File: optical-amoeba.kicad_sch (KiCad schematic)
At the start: 5 parts, among them J1 Conn_01x08_Male, Q1 Q_Photo_NPN_CE

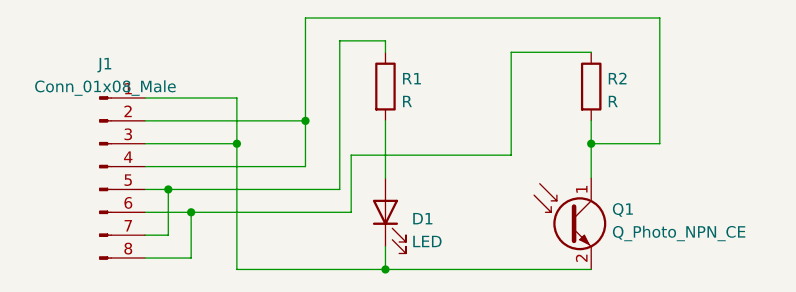
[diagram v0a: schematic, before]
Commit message: Add jlcpcb gerber and assembly files
M  OpticalSymbols_Library.kicad_sym
A  jlcpcb/gerber/optical-amoeba-B_Cu.gbl
A  jlcpcb/gerber/optical-amoeba-B_Mask.gbs
A  jlcpcb/gerber/optical-amoeba-B_Paste.gbp
A  jlcpcb/gerber/optical-amoeba-B_Silkscreen.gbo
A  jlcpcb/gerber/optical-amoeba-Edge_Cuts.gm1
A  jlcpcb/gerber/optical-amoeba-F_Cu.gtl
A  jlcpcb/gerber/optical-amoeba-F_Mask.gts
A  jlcpcb/gerber/optical-amoeba-F_Paste.gtp
A  jlcpcb/gerber/optical-amoeba-F_Silkscreen.gto
A  jlcpcb/gerber/optical-amoeba-NPTH-drl_map.gbr
A  jlcpcb/gerber/optical-amoeba-NPTH.drl
A  jlcpcb/gerber/optical-amoeba-PTH-drl_map.gbr
A  jlcpcb/gerber/optical-amoeba-PTH.drl
M  optical-amoeba.kicad_pcb
M  optical-amoeba.kicad_prl
M  optical-amoeba.kicad_sch
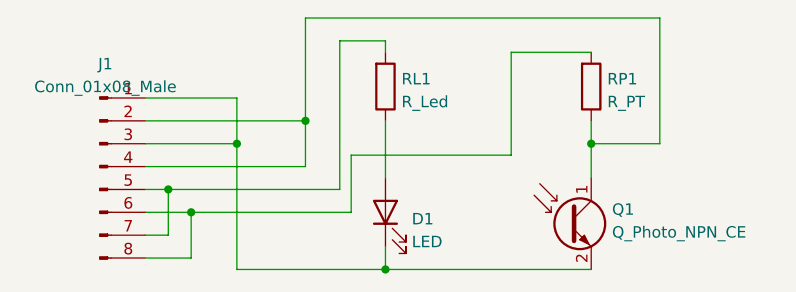
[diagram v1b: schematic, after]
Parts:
- removed R1: R, Resistor_SMD:R_0603_1608Metric, symbol Device:R
- removed R2: R, Resistor_SMD:R_0805_2012Metric, symbol Device:R
- added RL1: R_Led, Resistor_SMD:R_0603_1608Metric, symbol OpticalSymbols_Library:R_Led
- added RP1: R_PT, Resistor_SMD:R_0805_2012Metric, symbol OpticalSymbols_Library:R_PT
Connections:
- net at J1.2 (Pin_2), J1.4 (Pin_4), Q1.1 (C): now also RP1.2
- net at J1.5 (Pin_5), J1.7 (Pin_7): now also RL1.1
- net at J1.6 (Pin_6), J1.8 (Pin_8): now also RP1.1
- net at D1.2 (A): now also RL1.2
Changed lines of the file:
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@@
     (pin "8")
-  )
-  (symbol (lib_id "Device:R") (at 100.33 67.31 0) (unit 1)
-    (in_bom yes) (on_board yes) (fields_autoplaced)
-    (property "Reference" "R1" (id 0) (at 102.108 66.4753 0)
-      (effects (font (size 1.27 1.27)) (justify left))
-    )
-    (property "Value" "R" (id 1) (at 102.108 69.0122 0)
-      (effects (font (size 1.27 1.27)) (justify left))
-    )
-    (property "Footprint" "Resistor_SMD:R_0603_1608Metric" (id 2) (at 98.552 67.31 90)
-      (effects (font (size 1.27 1.27)) hide)
-    )
-    (property "Datasheet" "~" (id 3) (at 100.33 67.31 0)
-      (effects (font (size 1.27 1.27)) hide)
-    )
-    (property "JLC" "0603" (id 4) (at 100.33 67.31 0)
-      (effects (font (size 1.27 1.27)) hide)
-    )
-    (property "LCSC" "C4190" (id 5) (at 100.33 67.31 0)
-      (effects (font (size 1.27 1.27)) hide)
-    )
-    (pin "1")
-    (pin "2")
   )
   (symbol (lib_id "Device:Q_Photo_NPN_CE") (at 120.65 82.55 0) (unit 1)
@@
     (property "LCSC" "C264383" (id 5) (at 120.65 82.55 0)
       (effects (font (size 1.27 1.27)) hide)
+    )
+    (pin "1")
+    (pin "2")
+  )
+  (symbol (lib_id "OpticalSymbols_Library:R_PT") (at 123.19 67.31 0) (unit 1)
+    (in_bom yes) (on_board yes) (fields_autoplaced)
+    (property "Reference" "RP1" (id 0) (at 124.968 66.4753 0)
+      (effects (font (size 1.27 1.27)) (justify left))
+    )
+    (property "Value" "R_PT" (id 1) (at 124.968 69.0122 0)
+      (effects (font (size 1.27 1.27)) (justify left))
+    )
+    (property "Footprint" "Resistor_SMD:R_0805_2012Metric" (id 2) (at 124.46 73.66 90)
+      (effects (font (size 1.27 1.27)) (justify left) hide)
+    )
+    (property "Datasheet" "~" (id 3) (at 123.19 68.58 0)
+      (effects (font (size 1.27 1.27)) hide)
+    )
+    (property "JLC" "0805-2012" (id 4) (at 120.65 71.12 0)
+      (effects (font (size 0.5 0.5)) hide)
+    )
+    (property "LCSC" "C17713" (id 5) (at 127 63.5 0)
+      (effects (font (size 0.5 0.5)) hide)
+    )
+    (pin "1")
+    (pin "2")
+  )
+  (symbol (lib_id "OpticalSymbols_Library:R_Led") (at 100.33 67.31 0) (unit 1)
+    (in_bom yes) (on_board yes) (fields_autoplaced)
+    (property "Reference" "RL1" (id 0) (at 102.108 66.4753 0)
+      (effects (font (size 1.27 1.27)) (justify left))
+    )
+    (property "Value" "R_Led" (id 1) (at 102.108 69.0122 0)
+      (effects (font (size 1.27 1.27)) (justify left))
+    )
+    (property "Footprint" "Resistor_SMD:R_0603_1608Metric" (id 2) (at 101.6 73.66 90)
+      (effects (font (size 1.27 1.27)) (justify left) hide)
+    )
+    (property "Datasheet" "~" (id 3) (at 100.33 68.58 0)
+      (effects (font (size 1.27 1.27)) hide)
+    )
+    (property "JLC" "0603-1608" (id 4) (at 104.14 71.12 0)
+      (effects (font (size 0.5 0.5)) hide)
+    )
+    (property "LCSC" "C4190" (id 5) (at 104.14 63.5 0)
+      (effects (font (size 0.5 0.5)) hide)
     )
     (pin "1")
@@
     (pin "2")
   )
-  (symbol (lib_id "Device:R") (at 123.19 67.31 0) (unit 1)
-    (in_bom yes) (on_board yes) (fields_autoplaced)
-    (property "Reference" "R2" (id 0) (at 124.968 66.4753 0)
-      (effects (font (size 1.27 1.27)) (justify left))
-    )
-    (property "Value" "R" (id 1) (at 124.968 69.0122 0)
-      (effects (font (size 1.27 1.27)) (justify left))
-    )
-    (property "Footprint" "Resistor_SMD:R_0805_2012Metric" (id 2) (at 121.412 67.31 90)
-      (effects (font (size 1.27 1.27)) hide)
-    )
-    (property "Datasheet" "~" (id 3) (at 123.19 67.31 0)
-      (effects (font (size 1.27 1.27)) hide)
-    )
-    (property "JLC" "0805" (id 4) (at 123.19 67.31 0)
-      (effects (font (size 1.27 1.27)) hide)
-    )
-    (property "LCSC" "C17713" (id 5) (at 123.19 67.31 0)
-      (effects (font (size 1.27 1.27)) hide)
-    )
-    (pin "1")
-    (pin "2")
-  )
   (sheet_instances
     (path "/" (page "1"))
@@
       (reference "Q1") (unit 1) (value "Q_Photo_NPN_CE") (footprint "Optical_Parts:Everlight_PT_PT12-21C_TR8")
     )
-    (path "/23503685-6c48-4b6b-a5a1-d4b81440ce50"
-      (reference "R1") (unit 1) (value "R") (footprint "Resistor_SMD:R_0603_1608Metric")
+    (path "/ae276f22-adb9-4929-9ca1-9c2610beeee5"
+      (reference "RL1") (unit 1) (value "R_Led") (footprint "Resistor_SMD:R_0603_1608Metric")
     )
-    (path "/f10b485f-7f48-45c9-945a-aa2d898f983c"
-      (reference "R2") (unit 1) (value "R") (footprint "Resistor_SMD:R_0805_2012Metric")
+    (path "/5a77a3a7-0cd1-4017-977f-0774e58d08ed"
+      (reference "RP1") (unit 1) (value "R_PT") (footprint "Resistor_SMD:R_0805_2012Metric")
     )
   )
